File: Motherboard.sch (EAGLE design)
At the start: 44 parts, among them IC1 MAX6954AAX+, IC2 MCP23017SO, U6 MAX3232

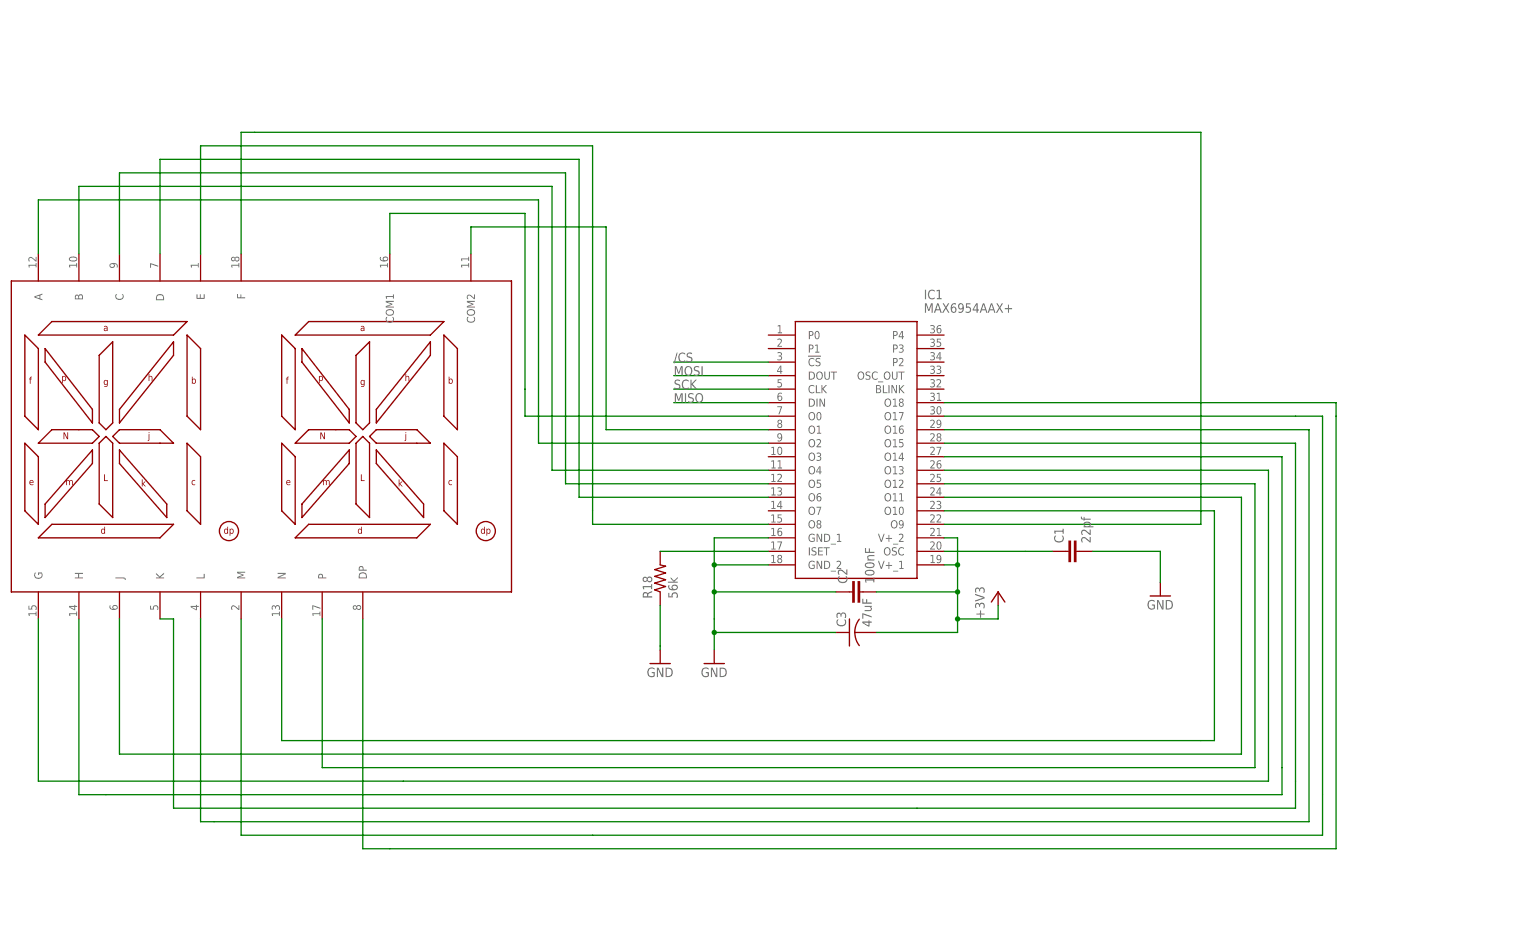
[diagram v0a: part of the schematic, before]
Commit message: well it works now
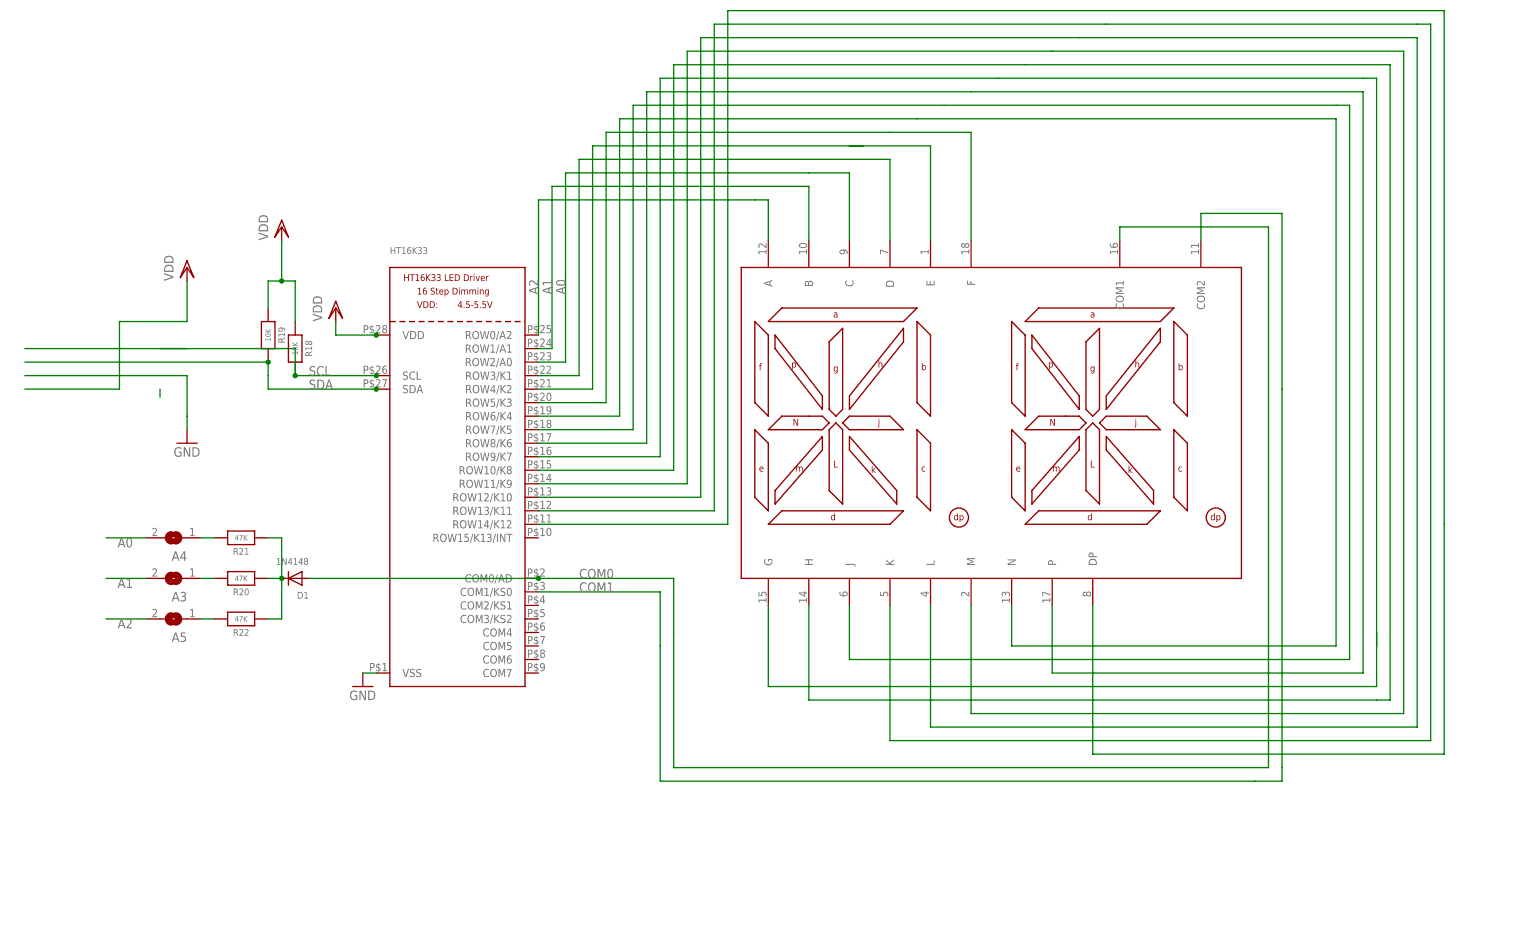
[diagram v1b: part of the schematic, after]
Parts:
- removed C1: 22pf, SparkFun-Capacitors:1.0UF-0805-25V-(+80/-20%)
- removed C2: 100nF, SparkFun-Capacitors:1.0UF-0805-25V-(+80/-20%)
- removed C3: 47uF, adafruit:C-USC1206
- removed IC1: MAX6954AAX+, SamacSys_Parts:MAX6954AAX+
- added A3, A4, A5: (no value), microbuilder:SOLDERJUMPERREFLOW_NOPASTE
- added D1: 1N4148, adafruit:DIODESOD-323F
- added HT16K33: (no value), microbuilder:HT16K33_SOP28_SKINNY
- added R19: 10K, microbuilder:RESISTOR0805_NOOUTLINE
- added R20, R21, R22: 47K, microbuilder:RESISTOR0805_NOOUTLINE
- R18: value 56k -> 10K; device resistor:R-US_M0805 -> microbuilder:RESISTOR0805_NOOUTLINE
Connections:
- removed net N$13: IC1.O15, U$1.K
- removed net N$14: IC1.O16, U$1.L
- removed net N$15: IC1.O17, U$1.M
- removed net N$16: IC1.O18, U$1.DP
- removed net N$17: IC1.O1, U$1.COM2
- removed net N$30: C1.1, IC1.OSC
- removed net N$31: IC1.ISET, R18.2
- new net A0: A4.2, HT16K33.ROW2/A0, U$1.C
- new net A1: A3.2, HT16K33.ROW1/A1, U$1.B
- new net A2: A5.2, HT16K33.ROW0/A2, U$1.A
- new net COM0: D1.A, HT16K33.COM0/AD, U$1.COM1
- new net COM1: HT16K33.COM1/KS0, U$1.COM2
- new net N$32: HT16K33.ROW11/K9, U$1.M
- new net N$33: HT16K33.ROW12/K10, U$1.L
- new net N$34: HT16K33.ROW13/K11, U$1.K
- new net N$35: HT16K33.ROW14/K12, U$1.DP
- new net VDD: HT16K33.VDD, R18.1, R19.1
- net +3V3: no longer C2.2, C3.2, IC1.V+_1, IC1.V+_2
- net /CS: no longer IC1.!CS
- net GND: now also HT16K33.VSS; no longer C1.2, C2.1, C3.1, IC1.GND_1, IC1.GND_2, R18.1
- net MISO: no longer IC1.DIN
- net MOSI: no longer IC1.DOUT
- net N$1: now also A3.1, R20.2; no longer IC1.O0, U$1.COM1
- net N$10: now also HT16K33.ROW8/K6; no longer IC1.O12
- net N$11: now also HT16K33.ROW9/K7; no longer IC1.O13
- net N$12: now also HT16K33.ROW10/K8; no longer IC1.O14
- net N$2: now also A4.1, R21.2; no longer IC1.O2, U$1.A
- net N$3: now also HT16K33.ROW3/K1, U$1.D; no longer IC1.O4, U$1.B
- net N$4: now also HT16K33.ROW4/K2, U$1.E; no longer IC1.O5, U$1.C
- net N$5: now also HT16K33.ROW5/K3, U$1.F; no longer IC1.O6, U$1.D
- net N$6: now also HT16K33.ROW6/K4, U$1.N; no longer IC1.O8, U$1.E
- net N$7: now also HT16K33.ROW7/K5, U$1.J; no longer IC1.O9, U$1.F
- net N$8: now also D1.C, R20.1, R21.1, R22.1; no longer IC1.O10, U$1.N
- net N$9: now also A5.1, R22.2; no longer IC1.O11, U$1.J
- net SCK: no longer IC1.CLK
- net SCL: now also HT16K33.SCL, R18.2
- net SDA: now also HT16K33.SDA, R19.2
